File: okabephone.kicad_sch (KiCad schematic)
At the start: 41 parts, among them J1 Micro_SD_Card_Det1, M1 Motor_DC, Q1 AO3400A, SW1 SW_Push, SW10 SW_Push, SW11 SW_Push, SW12 SW_Push, SW13 SW_Push, SW14 SW_Push, SW15 SW_Push, SW16 SW_Push, SW17 SW_Push, SW18 SW_Push, SW19 SW_Push, SW2 SW_Push, SW3 SW_Push, SW4 SW_Push, SW5 SW_Push, SW6 SW_Push, SW7 SW_Push, SW8 SW_Push, SW9 SW_Push, U1 MCP23017_ML, U2 ESP32-S3-WROOM-1, U6 PCF8563T, Y1 32.768kHz

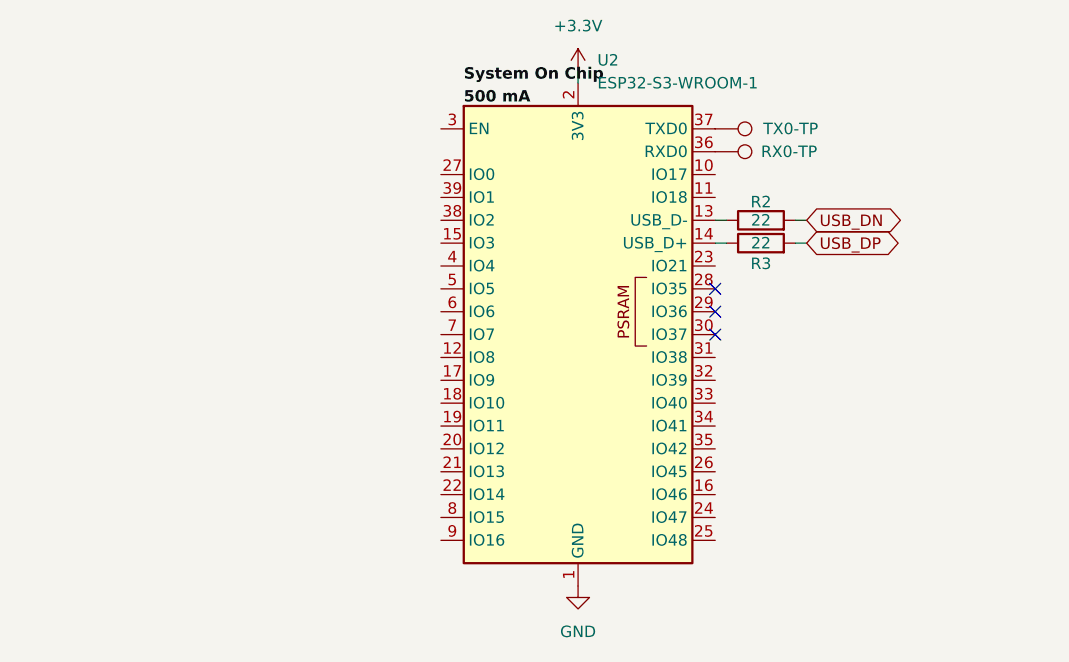
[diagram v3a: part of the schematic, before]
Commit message: spi joke
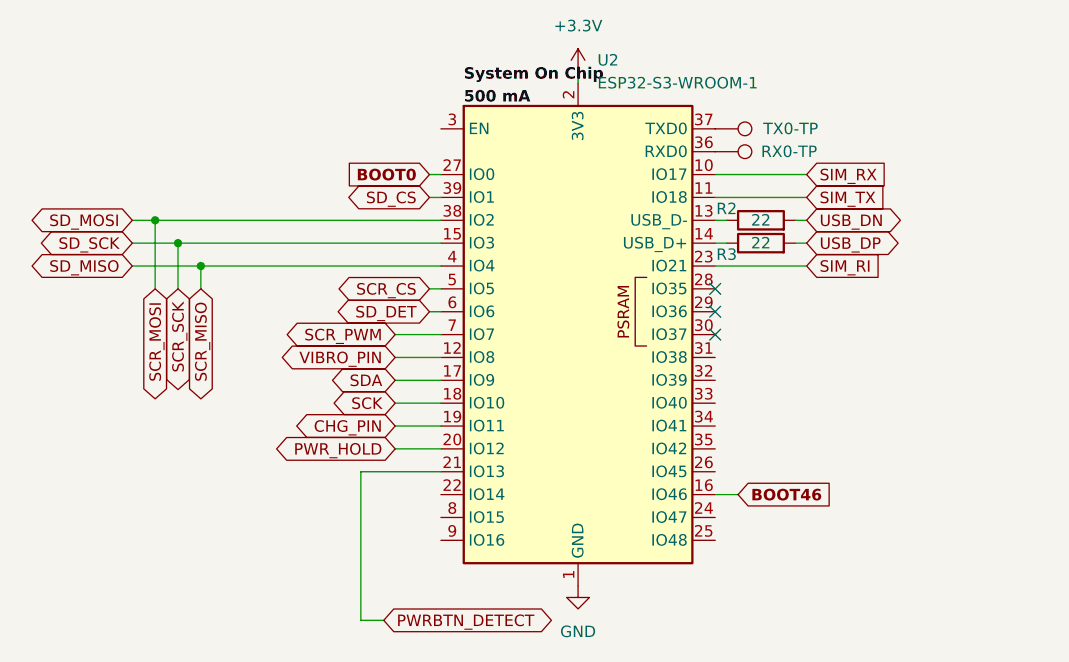
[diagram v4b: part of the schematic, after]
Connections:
- net SD_MISO is gone; now on net SCR_MISO: J1.7 (DAT0), R12.2
- net SD_MOSI is gone; now on net SCR_MOSI: J1.3 (CMD), R11.2
- net SD_SCK is gone; now on net SCR_SCK: J1.5 (CLK)
- net SCK: now also U2.18 (IO10)
- net SDA: now also U2.17 (IO9)
- net SD_CS: now also U2.39 (IO1)
- net SD_DET: now also U2.6 (IO6)
- net VIBRO_PIN: now also U2.12 (IO8)
- net SIM_RX: now reaches U2.10 (IO17)
- net SIM_TX: now reaches U2.11 (IO18)
- net SCR_SCK: now reaches U2.15 (IO3)
- net BOOT46: now reaches U2.16 (IO46)
- net CHG_PIN: now reaches U2.19 (IO11)
- net PWR_HOLD: now reaches U2.20 (IO12)
- net PWRBTN_DETECT: now reaches U2.21 (IO13)
- net SIM_RI: now reaches U2.23 (IO21)
- net BOOT0: now reaches U2.27 (IO0)
- net SCR_MOSI: now reaches U2.38 (IO2)
- net SCR_MISO: now reaches U2.4 (IO4)
- net SCR_CS: now reaches U2.5 (IO5)
- net SCR_PWM: now reaches U2.7 (IO7)

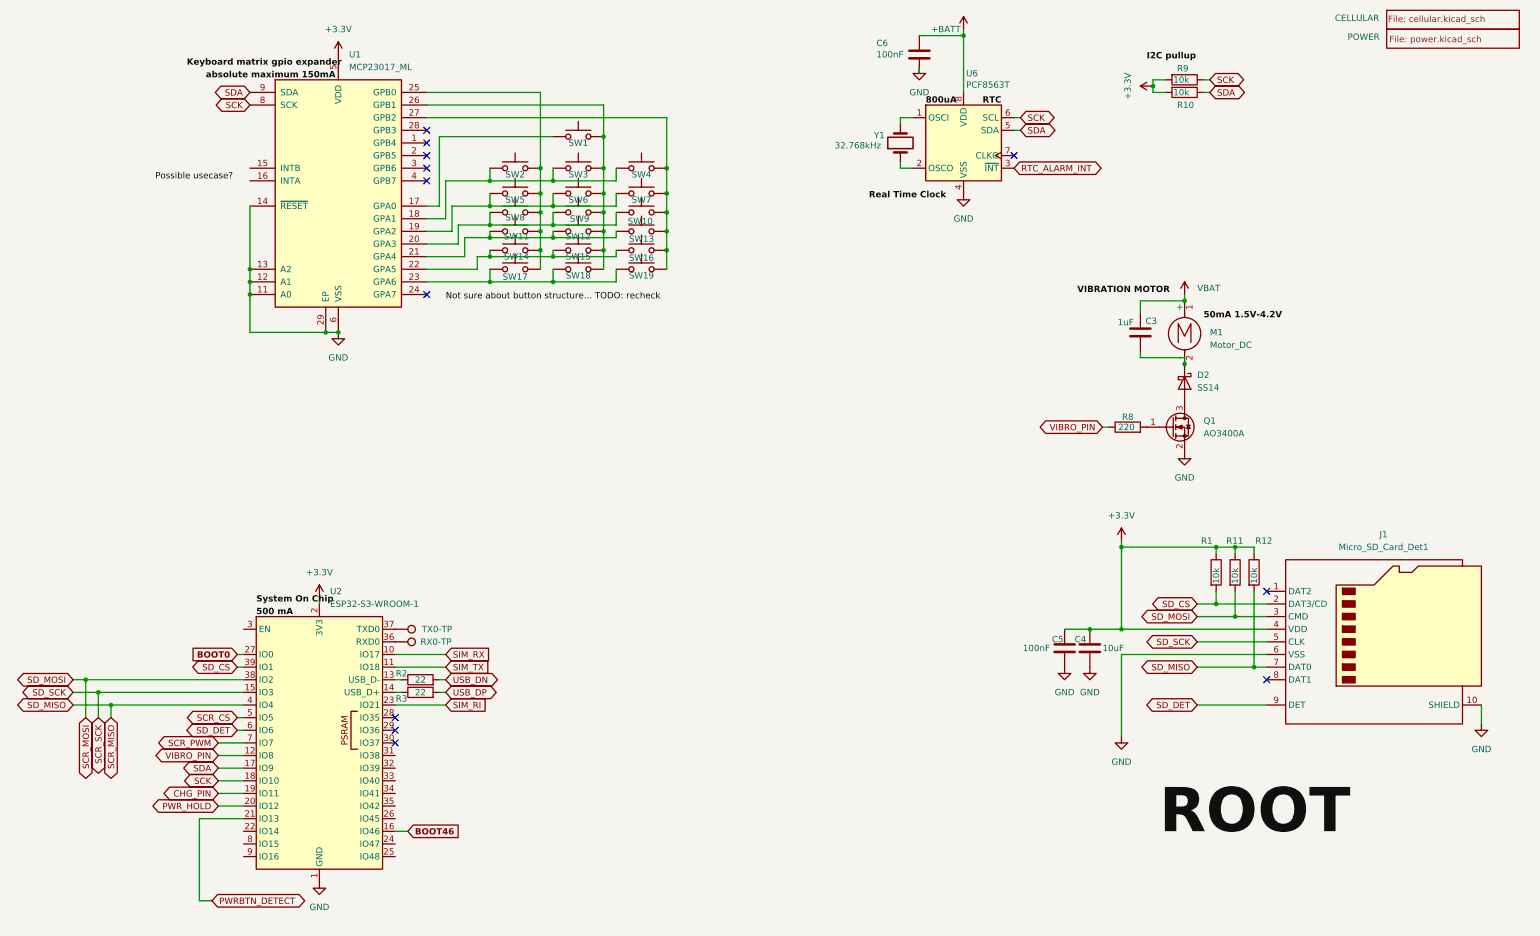
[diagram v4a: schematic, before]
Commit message: buck converter
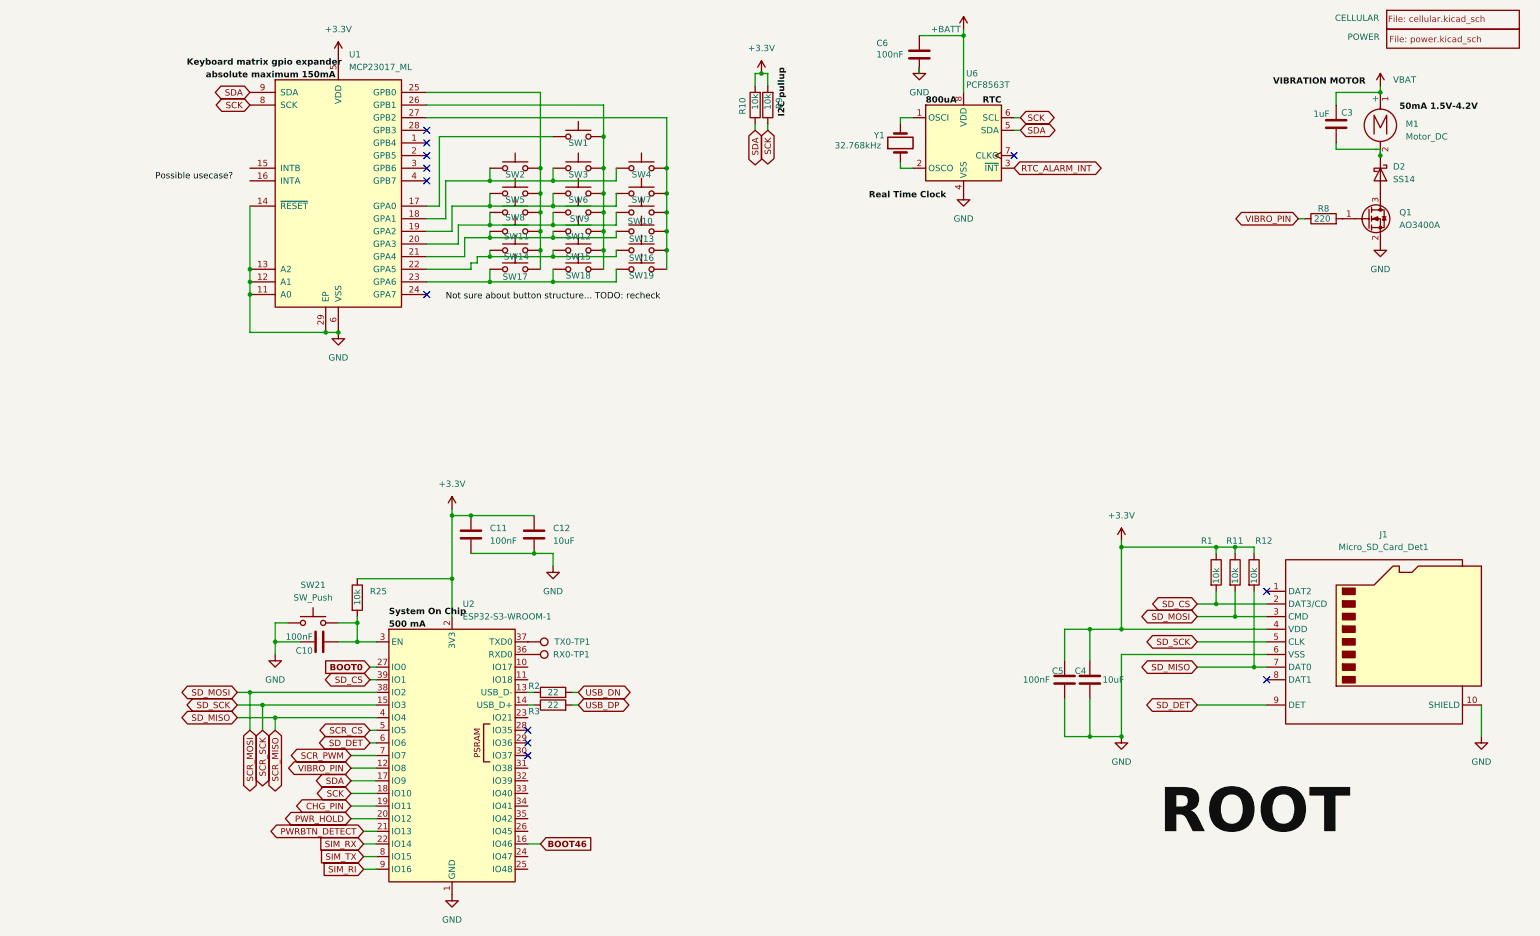
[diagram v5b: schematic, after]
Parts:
- added C10, C11: 100nF, symbol Device:C
- added C12: 10uF, symbol Device:C
- added R25: 10k, symbol Device:R
- added SW21: SW_Push, symbol Switch:SW_Push
- renumbered RX0-TP to RX0-TP1, TX0-TP to TX0-TP1
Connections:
- net +3.3V: now also C11.1, C12.1, R25.1
- net GND: now also C10.1, C11.2, C12.2, SW21.1
- net SIM_RI: now also U2.9 (IO16); no longer U2.23 (IO21)
- net SIM_RX: now also U2.22 (IO14); no longer U2.10 (IO17)
- net SIM_TX: now also U2.8 (IO15); no longer U2.11 (IO18)
- net at U2.3 (EN): now also C10.2, R25.2, SW21.2
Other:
- moved on the sheet: C3, C4, C5, D2, M1, Q1, R10, R2, R3, R8, R9, RX0-TP1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

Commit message: eee:
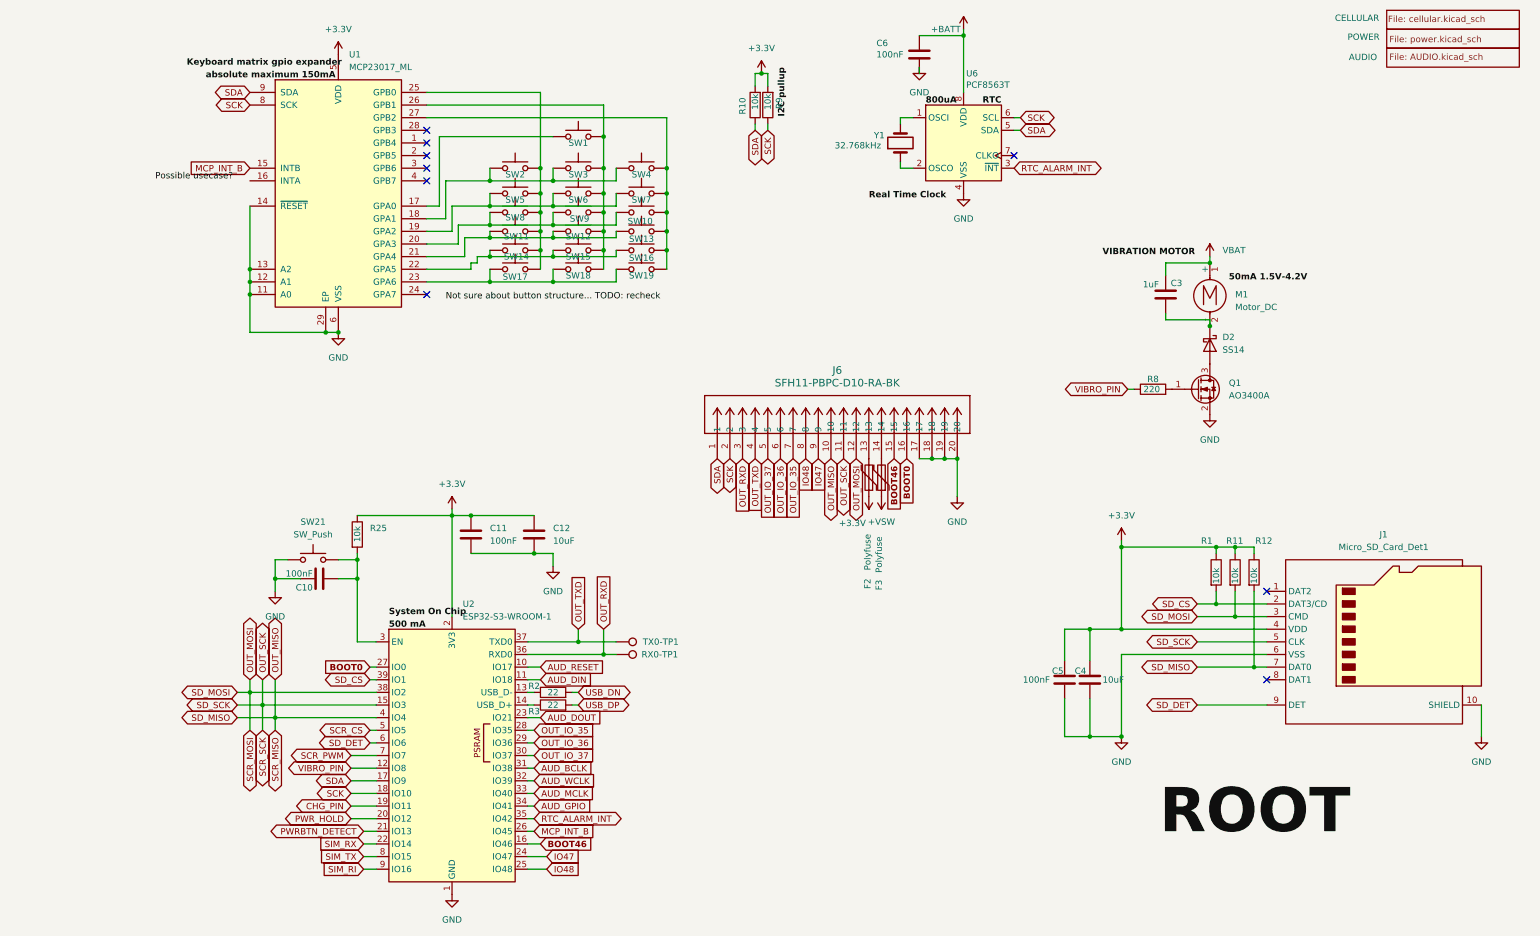
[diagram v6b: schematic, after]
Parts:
- added F2, F3: Polyfuse, symbol Device:Polyfuse
- added J6: SFH11-PBPC-D10-RA-BK, CONN20_D10-RA-BK_SUL, symbol 20PIN Connector:SFH11-PBPC-D10-RA-BK
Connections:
- net +3.3V: now also F2.1
- net BOOT0: now also J6.16
- net BOOT46: now also J6.15
- net GND: now also J6.17, J6.18, J6.19, J6.20
- net RTC_ALARM_INT: now also U2.35 (IO42)
- net SCK: now also J6.2
- net SDA: now also J6.1
- net AUD_RESET: now reaches U2.10 (IO17)
- net AUD_DIN: now reaches U2.11 (IO18)
- net AUD_DOUT: now reaches U2.23 (IO21)
- net IO47: now reaches U2.24 (IO47)
- net IO47: now also J6.9
- net IO48: now reaches U2.25 (IO48)
- net IO48: now also J6.8
- net MCP_INT_B: now reaches U2.26 (IO45)
- net MCP_INT_B: now also U1.15 (INTB)
- net OUT_IO_35: now reaches U2.28 (IO35)
- net OUT_IO_35: now also J6.7
- net OUT_IO_36: now reaches U2.29 (IO36)
- net OUT_IO_36: now also J6.6
- net OUT_IO_37: now reaches U2.30 (IO37)
- net OUT_IO_37: now also J6.5
- net AUD_BCLK: now reaches U2.31 (IO38)
- net AUD_WCLK: now reaches U2.32 (IO39)
- net AUD_MCLK: now reaches U2.33 (IO40)
- net AUD_GPIO: now reaches U2.34 (IO41)
- net OUT_RXD: now reaches RX0-TP1.1, U2.36 (RXD0)
- net OUT_RXD: now also J6.3
- net OUT_TXD: now reaches TX0-TP1.1, U2.37 (TXD0)
- net OUT_TXD: now also J6.4
- net SCR_MISO renamed OUT_MISO
- net OUT_MISO: now also J6.10
- net SCR_MOSI renamed OUT_MOSI
- net OUT_MOSI: now also J6.12
- net SCR_SCK renamed OUT_SCK
- net OUT_SCK: now also J6.11
- new net: F2.2, J6.13
- new net: F3.2, J6.14
- new net +VSW: F3.1
- no-connect marks 12 -> 9
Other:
- added sheet AUDIO (AUDIO.kicad_sch)
- moved on the sheet: C10, C3, D2, M1, Q1, R25, R8, RX0-TP1, SW21, TX0-TP1
